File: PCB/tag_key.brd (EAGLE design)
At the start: 44.5 x 29 mm, 7 parts

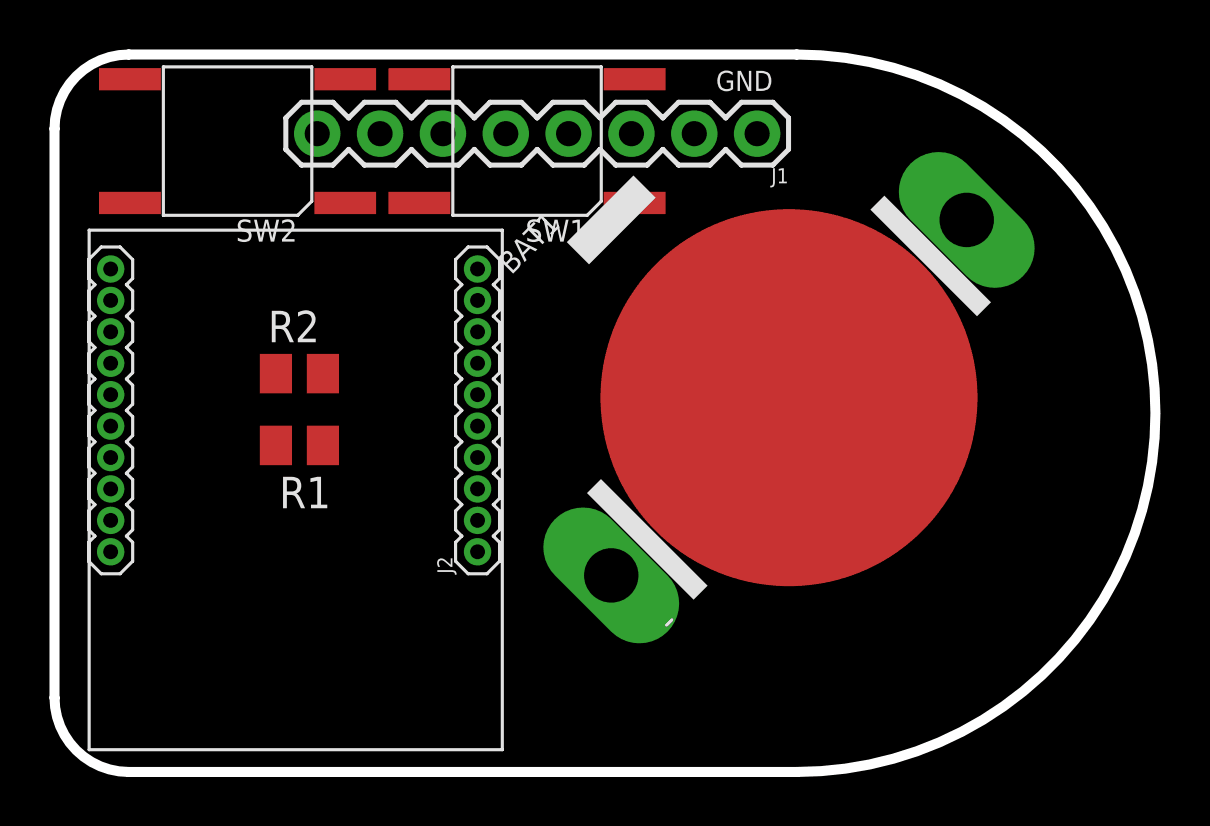
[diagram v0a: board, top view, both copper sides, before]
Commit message: tag,mail
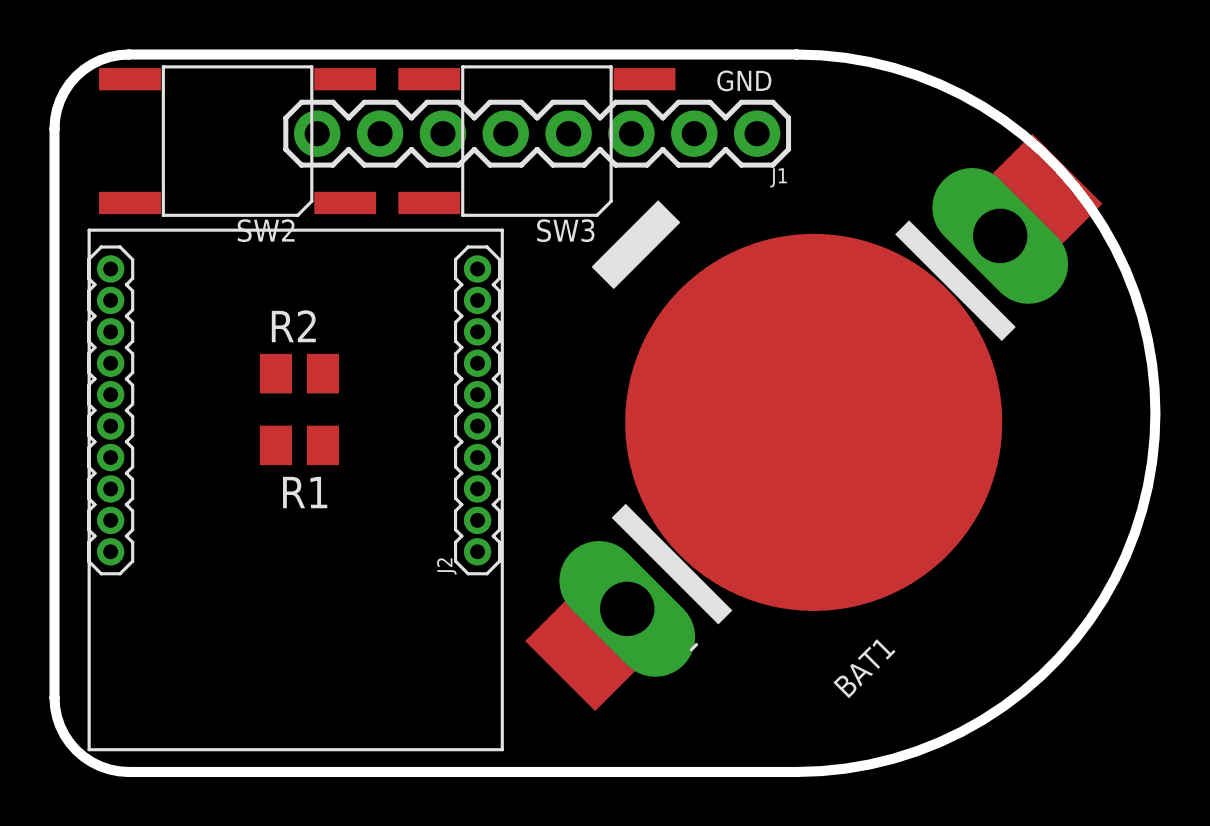
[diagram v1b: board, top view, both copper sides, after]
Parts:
- removed SW1: (no value), tag_key:SEEED-OPL-SWITCH_SW4-SMD-4.5-6.0X6.0X7.5MM
- added SW3: (no value), tag_key:SEEED-OPL-SWITCH_SW4-SMD-4.5-6.0X6.0_3LEG
- moved BAT1 1.41 mm to (27.7, 14.1)
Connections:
- net N$2: now also SW3.2; no longer SW1.2
- net P1.6: now also SW3.4; no longer SW1.4
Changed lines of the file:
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@@
 <setting verticaltext="up"/>
 </settings>
-<grid distance="0.1" unitdist="mm" unit="mm" style="lines" multiple="1" display="yes" altdistance="0.025" altunitdist="inch" altunit="inch"/>
+<grid distance="0.5" unitdist="mm" unit="mm" style="lines" multiple="1" display="yes" altdistance="0.025" altunitdist="inch" altunit="inch"/>
 <layers>
 <layer number="1" name="Top" color="4" fill="1" visible="yes" active="yes"/>
@@
 <element name="R1" library="tag_key" package="RESISTOR_M0805" value="" x="6.9" y="13.2" rot="R180"/>
 <element name="R2" library="tag_key" package="RESISTOR_M0805" value="" x="6.9" y="16.1"/>
-<element name="BAT1" library="tag_key" package="SEEED-OPL-CONNECTOR_BAT2P-20.32-CR2032" value="cr2032" x="26.68786875" y="15.1292875" rot="R45"/>
-<element name="SW1" library="tag_key" package="SEEED-OPL-SWITCH_SW4-SMD-4.5-6.0X6.0X7.5MM" value="" x="16.1" y="25.5" rot="R180"/>
+<element name="BAT1" library="tag_key" package="SEEED-OPL-CONNECTOR_BAT2P-20.32-CR2032" value="cr2032" x="27.68786875" y="14.1292875" rot="R45"/>
 <element name="SW2" library="tag_key" package="SEEED-OPL-SWITCH_SW4-SMD-4.5-6.0X6.0X7.5MM" value="" x="4.4" y="25.5" rot="R180"/>
 <element name="J1" library="tag_key" package="SPARKFUN-CONNECTORS_1X08" value="" x="25.4" y="25.8" rot="R180">
@@
 </element>
 <element name="J2" library="tag_key" package="SPARKFUN-CONNECTORS_1X11-1.27MM" value="" x="14.1" y="8.9" rot="R90"/>
+<element name="SW3" library="tag_key" package="SEEED-OPL-SWITCH_SW4-SMD-4.5-6.0X6.0_3LEG" value="" x="16.5" y="25.5" rot="R180"/>
 </elements>
 <signals>
@@
 <signal name="P1.6">
 <contactref element="J2" pad="5"/>
-<contactref element="SW1" pad="4"/>
-<wire x1="14.1" y1="13.98" x2="11.75" y2="28" width="0" layer="19" extent="1-1"/>
+<contactref element="SW3" pad="4"/>
+<wire x1="12.15" y1="28" x2="14.1" y2="13.98" width="0" layer="19" extent="1-1"/>
 </signal>
 <signal name="P1.5">
@@
 <contactref element="BAT1" pad="2"/>
 <contactref element="BAT1" pad="3"/>
-<wire x1="19.5036625" y1="7.94508125" x2="33.872071875" y2="22.313490625" width="0" layer="19" extent="1-1"/>
-<wire x1="14.1" y1="11.44" x2="19.5036625" y2="7.94508125" width="0" layer="19" extent="1-1"/>
+<wire x1="20.150109375" y1="6.591528125" x2="35.225625" y2="21.66704375" width="0" layer="19" extent="1-1"/>
+<wire x1="14.1" y1="11.44" x2="20.150109375" y2="6.591528125" width="0" layer="19" extent="1-1"/>
 </signal>
 <signal name="GND">
@@
 <contactref element="R2" pad="1"/>
 <contactref element="BAT1" pad="1"/>
-<wire x1="26.68786875" y1="15.1292875" x2="25.4" y2="25.8" width="0" layer="19" extent="1-1"/>
-<wire x1="14.1" y1="10.17" x2="26.68786875" y2="15.1292875" width="0" layer="19" extent="1-1"/>
+<wire x1="27.68786875" y1="14.1292875" x2="25.4" y2="25.8" width="0" layer="19" extent="1-1"/>
+<wire x1="14.1" y1="10.17" x2="27.68786875" y2="14.1292875" width="0" layer="19" extent="1-1"/>
 <wire x1="14.1" y1="8.9" x2="14.1" y2="10.17" width="0" layer="19" extent="1-1"/>
 <wire x1="7.85" y1="13.2" x2="14.1" y2="10.17" width="0" layer="19" extent="1-1"/>
@@
 <signal name="N$2">
 <contactref element="R1" pad="2"/>
-<contactref element="SW1" pad="2"/>
-<wire x1="5.95" y1="13.2" x2="11.75" y2="23" width="0" layer="19" extent="1-1"/>
+<contactref element="SW3" pad="2"/>
+<wire x1="12.15" y1="23" x2="5.95" y2="13.2" width="0" layer="19" extent="1-1"/>
 </signal>
 </signals>
